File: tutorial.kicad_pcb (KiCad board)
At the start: 2 copper layers, 175 x 164.8 mm, 68 parts

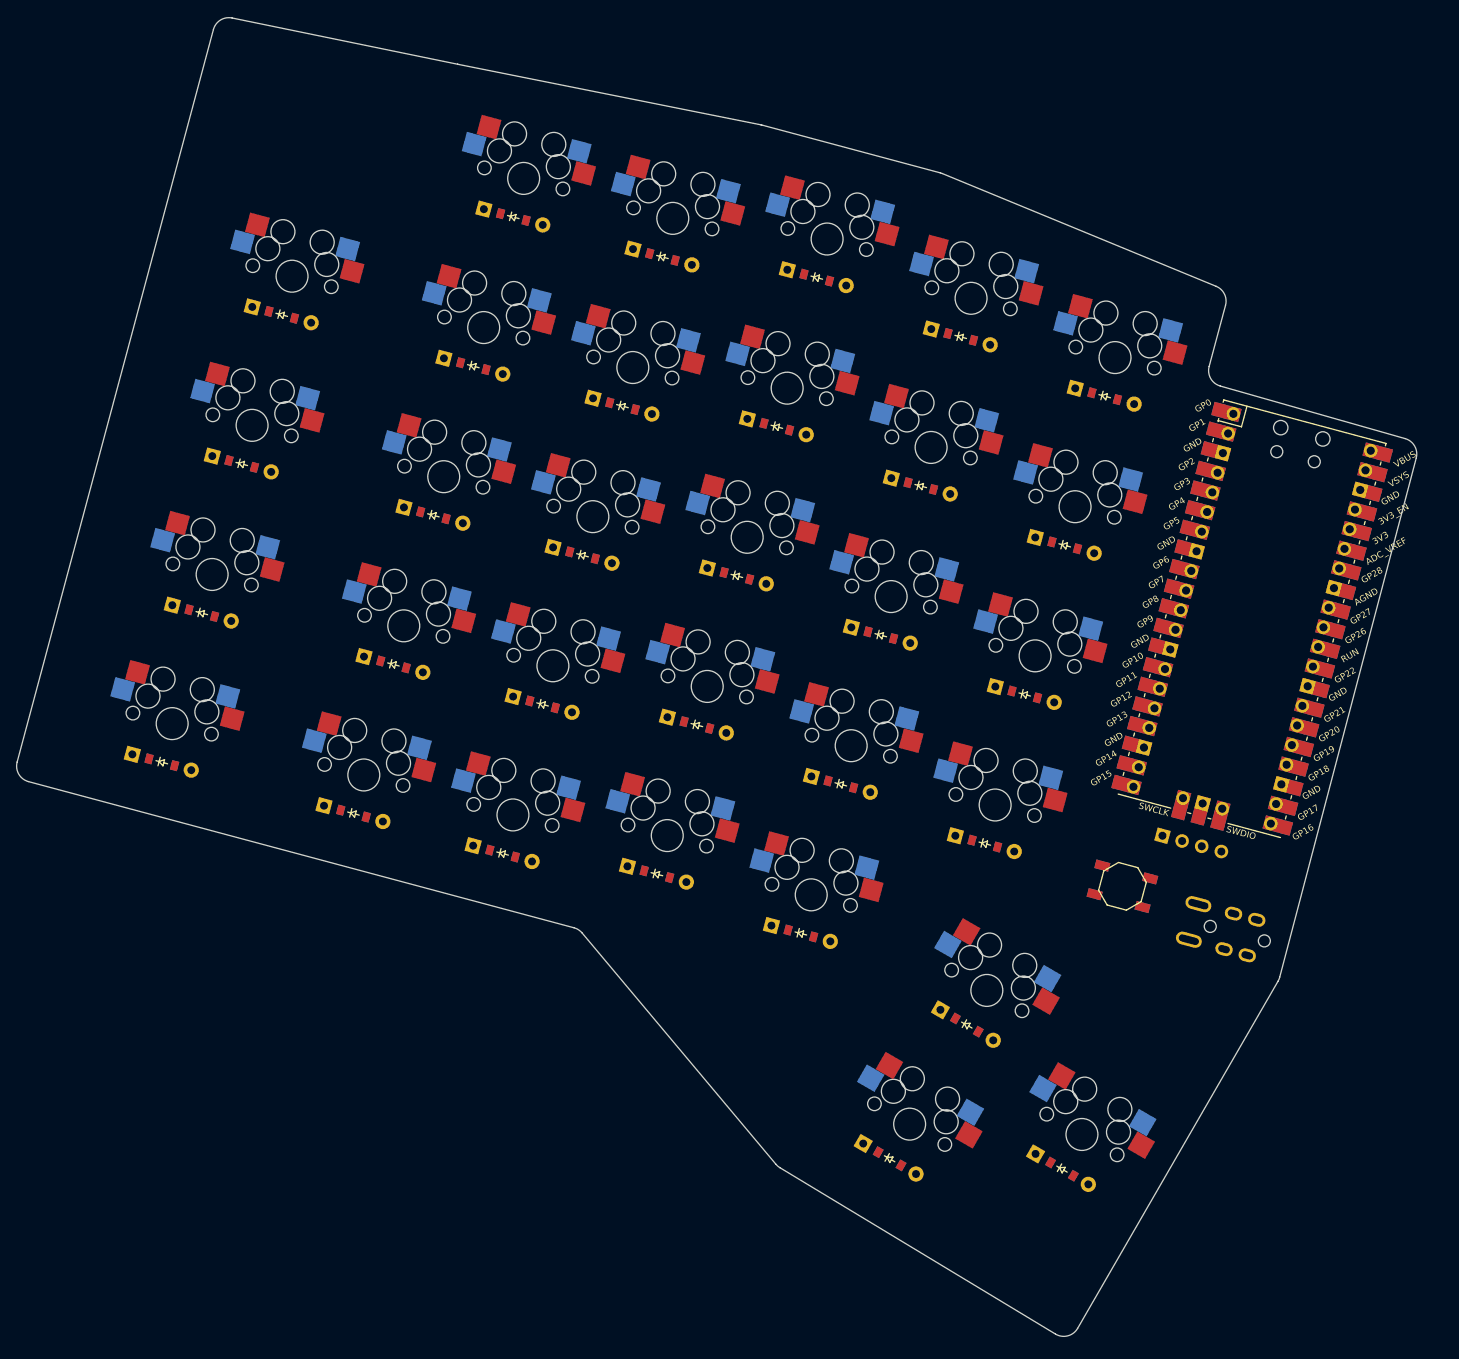
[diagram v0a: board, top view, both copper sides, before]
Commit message: ready to start routing
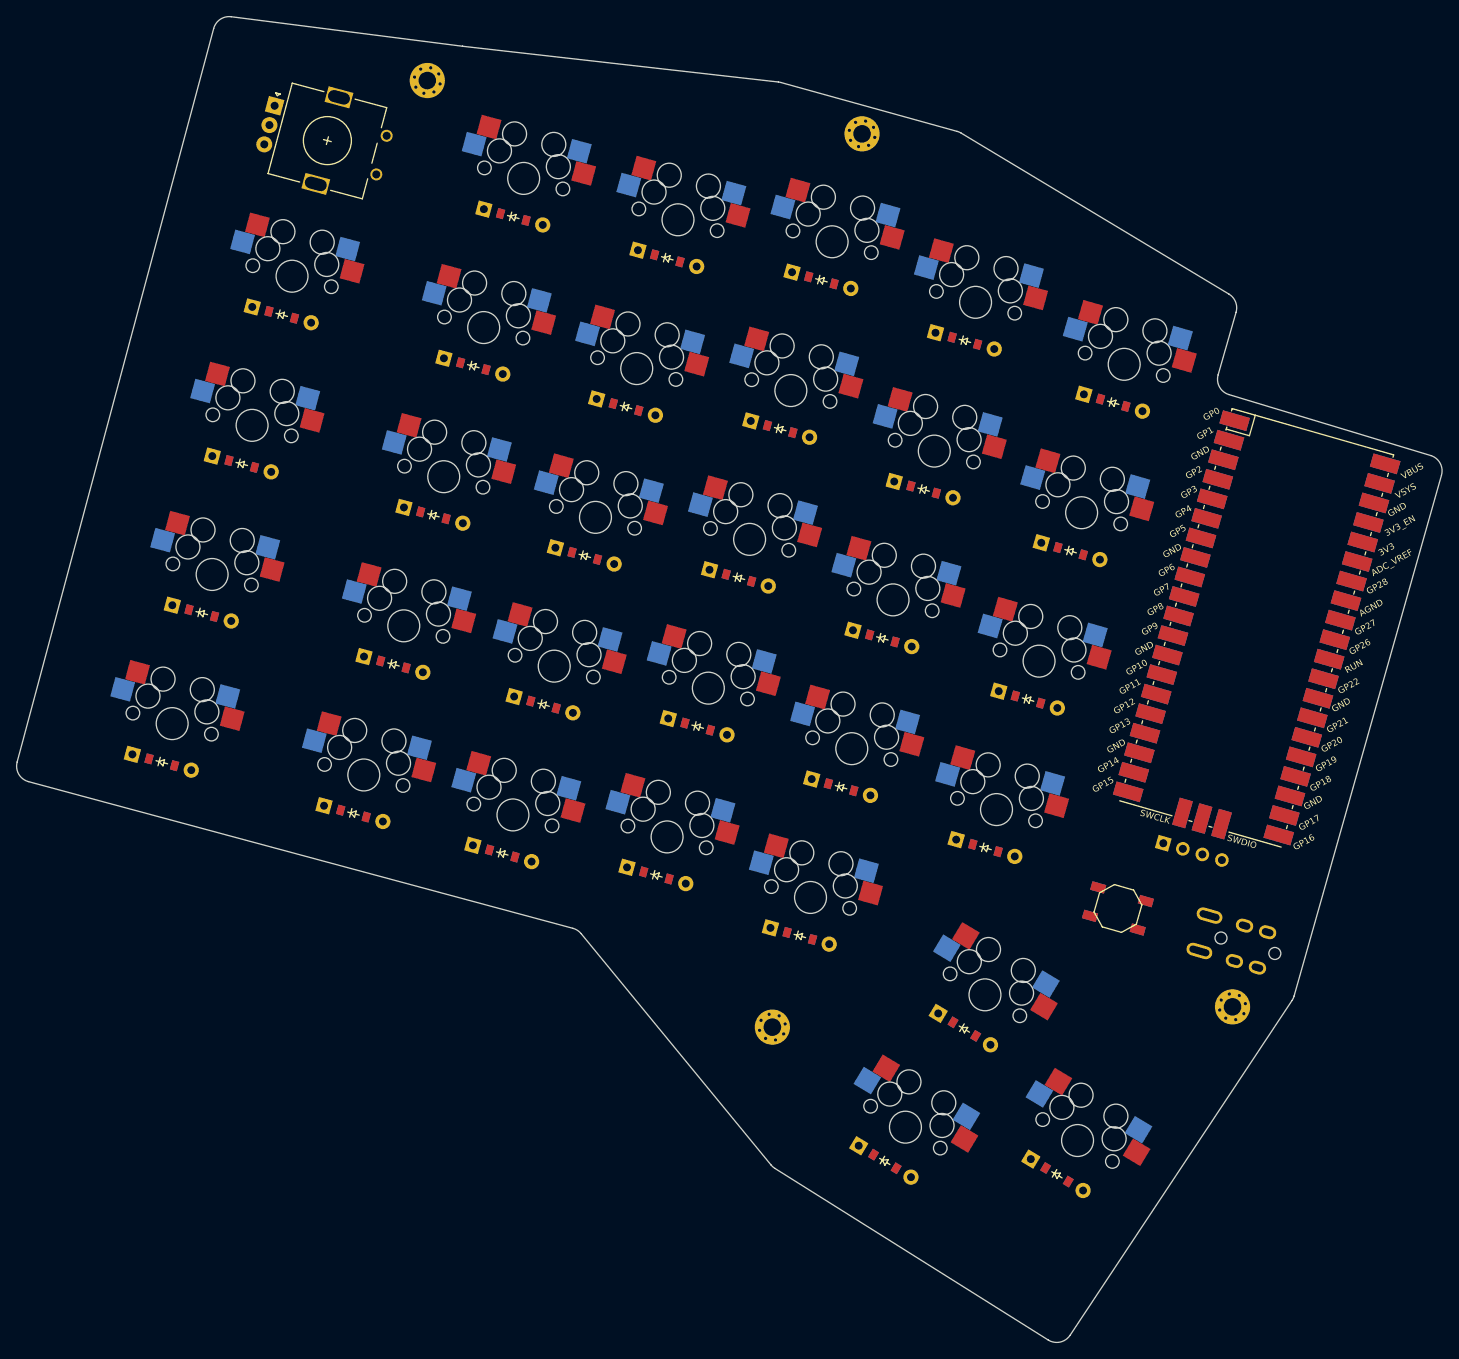
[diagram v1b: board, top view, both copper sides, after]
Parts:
- removed the _1 at (246.1, 152.0) (x2)
- added ROT1: , rotary_encoder, F.Cu at (130.6, 92.3)
- added _1 (x2): RPi_Pico_SMD_TH, RPi_Pico_SMD_TH, F.Cu at (246.6, 153.1)
- added _2: , MountingHole_2.2mm_M2_Pad_Via, F.Cu at (243.6, 200.5)
- added _3: , MountingHole_2.2mm_M2_Pad_Via, F.Cu at (186.1, 203.0)
- added _4: , MountingHole_2.2mm_M2_Pad_Via, F.Cu at (197.3, 91.3)
- added _5: , MountingHole_2.2mm_M2_Pad_Via, F.Cu at (143.0, 84.7)
- moved B1 2.83 mm to (229.3, 188.2), turned to -16 degrees
- moved B2 2.83 mm to (229.3, 188.2), turned to -16 degrees
- moved TRRS1 2.06 mm to (250.4, 194.2), turned to -106 degrees
- moved S28 1.42 mm to (230.1, 120.2), turned to -16 degrees
- moved D28 1.34 mm to (228.7, 125.0), turned to -16 degrees
- moved S27 1.11 mm to (224.7, 138.7), turned to -16 degrees
- moved OLED1 1.11 mm to (244.8, 181.2), turned to -106 degrees
- moved D27 1.04 mm to (223.4, 143.5), turned to -16 degrees
- moved D31 0.95 mm to (221.7, 221.5), turned to -31 degrees
- moved S31 0.93 mm to (224.2, 217.2), turned to -31 degrees
- moved S26 0.83 mm to (219.4, 157.3), turned to -16 degrees
- moved D26 0.76 mm to (218.0, 162.1), turned to -16 degrees
- moved S24 0.75 mm to (211.5, 112.4), turned to -15.5 degrees
- moved S19 0.72 mm to (193.6, 104.8), turned to -15.5 degrees
- moved D24 0.71 mm to (210.1, 117.2), turned to -15.5 degrees
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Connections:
- OLED1 pad 3: GP5 -> GP3
- OLED1 pad 4: GP4 -> GP2
- TRRS1 pad 3: P2 -> GP15
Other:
- board size 175 x 164.8 mm -> 178.2 x 165.7 mm
